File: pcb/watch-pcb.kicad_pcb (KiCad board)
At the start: 4 copper layers, 42 x 42 mm, 191 parts, among them J1 DAUGHTER, J2 USB_C_Receptacle, J3 ESP_ANT, J4 Micro_SD_Card, J5 ELV1411A, J6 TT143AMC12C, Q1 MMBT3904, Q2 MMBT3904, Q3 MMBT3904, Q4 MMBT3904, Q5 MMBT3904, Q6 MMBT3904, U1 ADP2108AUJ-1.8, U10 MAX30102, U11 TPS65631W, U12 DRV2605LYZFR, U13 LSM6DSV16XTR, U14 LIS3MDL, U2 TPS63021, U3 CP2102N-Axx-xQFN28, U4 BQ27427YZFR, U5 BQ25638, U6 ESP32-S3, U7 MX25LM51245GXDI00, U8 APS12808L-3OBMx, U9 TCA9535MRGER, Y1 32.768kHz, Y2 40MHz(10ppm)

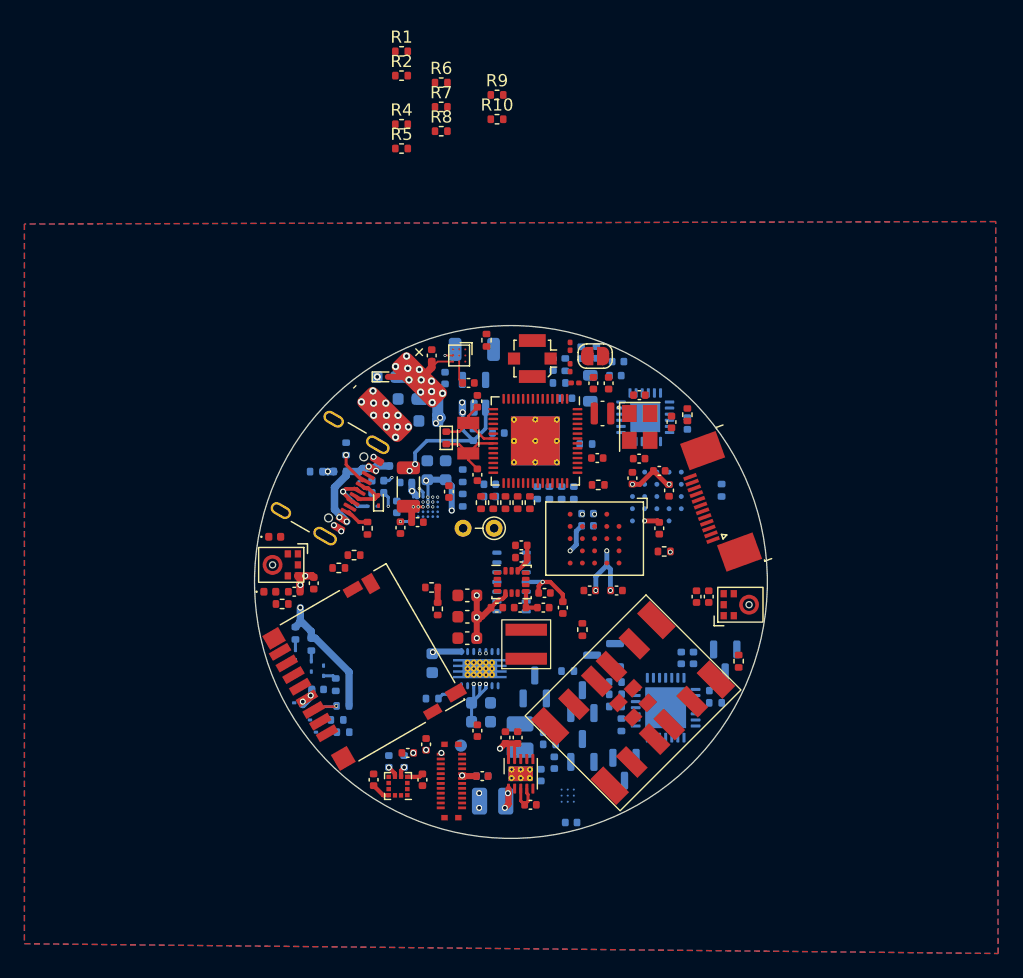
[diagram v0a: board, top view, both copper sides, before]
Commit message: made many changes, maybe switching to stm tho
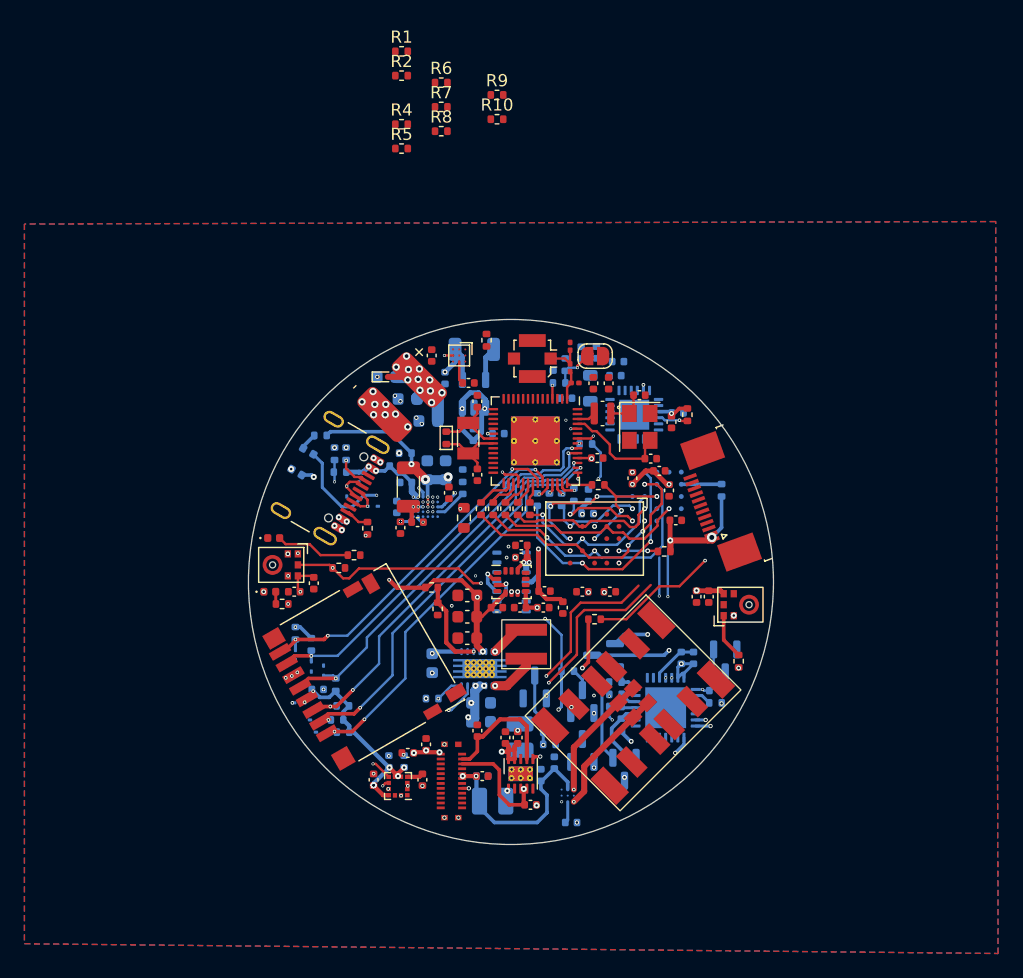
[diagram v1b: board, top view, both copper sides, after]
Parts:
- removed C34: 1uF, Capacitor_SMD:C_0402_1005Metric
- removed C37: 100nF, Capacitor_SMD:C_0402_1005Metric
- removed TP1: MTP_PWR, TestPoint:TestPoint_Pad_D1.0mm
- added R56: R, Resistor_SMD:R_0402_1005Metric, B.Cu at (101.2, 59.8)
- added R57: R, Resistor_SMD:R_0402_1005Metric, B.Cu at (108.1, 61.2)
- D4: moved to B.Cu
- TH1: footprint Resistor_THT:R_Axial_DIN0204_L3.6mm_D1.6mm_P2.54mm_Vertical -> Resistor_SMD:R_0603_1608Metric
- moved D6 6.69 mm to (99.2, 62.8), turned to 150 degrees
- moved D7 6.64 mm to (100.2, 61.1), turned to 150 degrees
- moved D4 2.70 mm to (103.3, 64.4)
- moved TH1 2.61 mm to (112.9, 66.5), turned to 90 degrees
- moved C30 2.50 mm to (123.1, 64.7), turned to 90 degrees
- moved R17 2.09 mm to (102.3, 61.3), turned to -90 degrees
- moved C77 1.50 mm to (130.2, 66.8), turned to 0 degrees
- moved R28 1.31 mm to (123.6, 74.8), turned to 0 degrees
- moved C48 1.18 mm to (130.4, 58.0), turned to 180 degrees
- moved C42 0.95 mm to (128.2, 61.7), turned to 180 degrees
- moved U9 0.92 mm to (126.8, 58.1)
- moved C31 0.61 mm to (122.6, 72.6)
- moved R42 0.56 mm to (119.9, 65.1)
- moved R43 0.56 mm to (120.9, 65.1)
- moved C78 0.56 mm to (124.8, 72.6)
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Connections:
- C32 pad 2: Net-(U6-VDD3P3_CPU) -> +3V3
- C35 pad 2: Net-(U6-VDD3P3_CPU) -> +3V3
- D6 pad 2: +VSW -> Net-(D6-A)
- D7 pad 2: +VSW -> Net-(D7-A)
- J6 pad 24: Net-(J6-MTP_PWR) -> GND
- U6 pad 12: /IO/DISP_RST -> /IO/HBT_INT
- U6 pad 20: Net-(U6-VDD3P3_CPU) -> +3V3
- U6 pad 29: Net-(U6-VDD_SPI) -> unconnected-(U6-VDD_SPI-Pad29)
- U6 pad 36: /MCU and Memory/SD_CLK -> /MCU and Memory/SD_D1
- U6 pad 37: /MCU and Memory/SD_CMD -> /MCU and Memory/SD_D0
- U6 pad 44: /MCU and Memory/SD_D0 -> /MCU and Memory/SD_D2
- U6 pad 45: /MCU and Memory/SD_D1 -> /MCU and Memory/SD_D3
- U6 pad 46: Net-(U6-VDD3P3_CPU) -> +3V3
- U6 pad 47: /MCU and Memory/SD_D2 -> /MCU and Memory/SD_CMD
- U6 pad 48: /MCU and Memory/SD_D3 -> /MCU and Memory/SD_CLK
- U9 pad 4: /IO/HBT_INT -> /IO/DISP_RST
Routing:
- net +3V3: track 72.2 -> 217.1 mm, vias 28 -> 39
- net Net-(Q1-B): track 0.93 -> 43.7 mm, vias 1 -> 2
- net /MCU and Memory/EN: track 0.00 -> 39.2 mm, vias 0 -> 2
- net /MCU and Memory/EXT_IO14: track 2.56 -> 37.2 mm, vias 0 -> 4
- net /IO/MAG_DRDY: track 0.00 -> 33.0 mm, vias 0 -> 2
- net /MCU and Memory/SD_D3: track 0.87 -> 33.5 mm, vias 0 -> 3
- net /USB and Power/USB_DN: track 3.70 -> 36.3 mm, vias 0 -> 2
- net /MCU and Memory/SD_CLK: track 1.09 -> 33.6 mm, vias 0 -> 2
- net /MCU and Memory/SD_D2: track 0.87 -> 33.3 mm, vias 0 -> 3
- net /IO/MAG_INT: track 0.00 -> 32.3 mm, vias 0 -> 2
- net /USB and Power/ILIM: track 0.00 -> 31.9 mm, vias 0 -> 6
- net /MCU and Memory/SD_CMD: track 2.87 -> 33.9 mm, vias 1 -> 3
- net /IO/MIC_SD: track 0.00 -> 29.9 mm, vias 0 -> 3
- net /MCU and Memory/SD_D0: track 0.88 -> 29.4 mm, vias 0 -> 2
- net +1V8: track 5.05 -> 33.3 mm, vias 1 -> 2
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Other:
- board size 42 x 42 mm -> 43 x 43 mm
- copper layers 4 -> 6
